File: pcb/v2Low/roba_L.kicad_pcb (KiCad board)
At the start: 2 copper layers, 10.7 x 12.1 mm, 49 parts, among them SW1 SW_PUSH, SW10 SW_PUSH, SW11 SW_PUSH, SW12 SW_PUSH, SW13 SW_PUSH, SW14 SW_PUSH, SW15 SW_PUSH, SW16 SW_PUSH, SW17 SW_PUSH, SW18 SW_PUSH, SW19 SW_PUSH, SW2 SW_PUSH, SW20 SW_PUSH, SW21 SW_PUSH, SW22 SW_PUSH, SW23 SW_PUSH, SW24 SW_SPDT, SW3 SW_PUSH, SW4 SW_PUSH, SW5 SW_PUSH, SW6 SW_PUSH, SW7 SW_PUSH, SW8 SW_PUSH, SW9 SW_PUSH

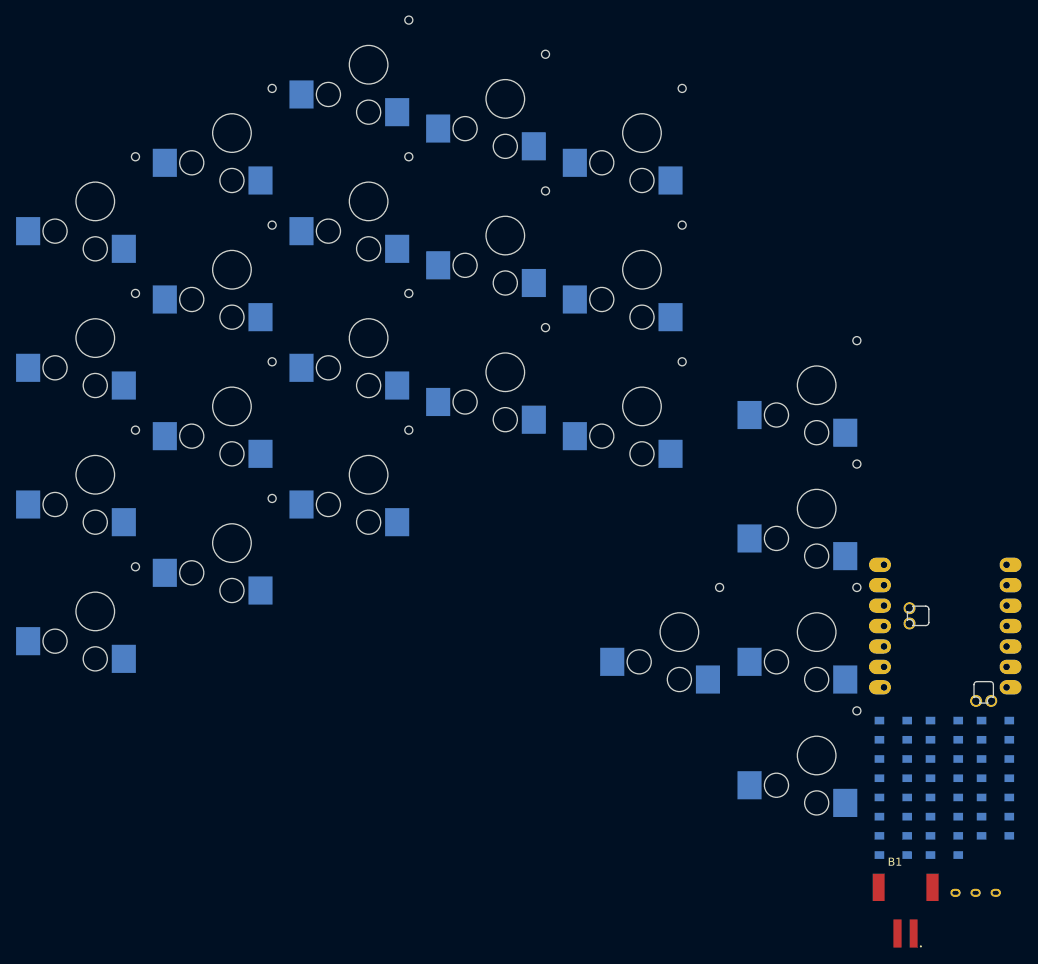
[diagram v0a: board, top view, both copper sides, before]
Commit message: save
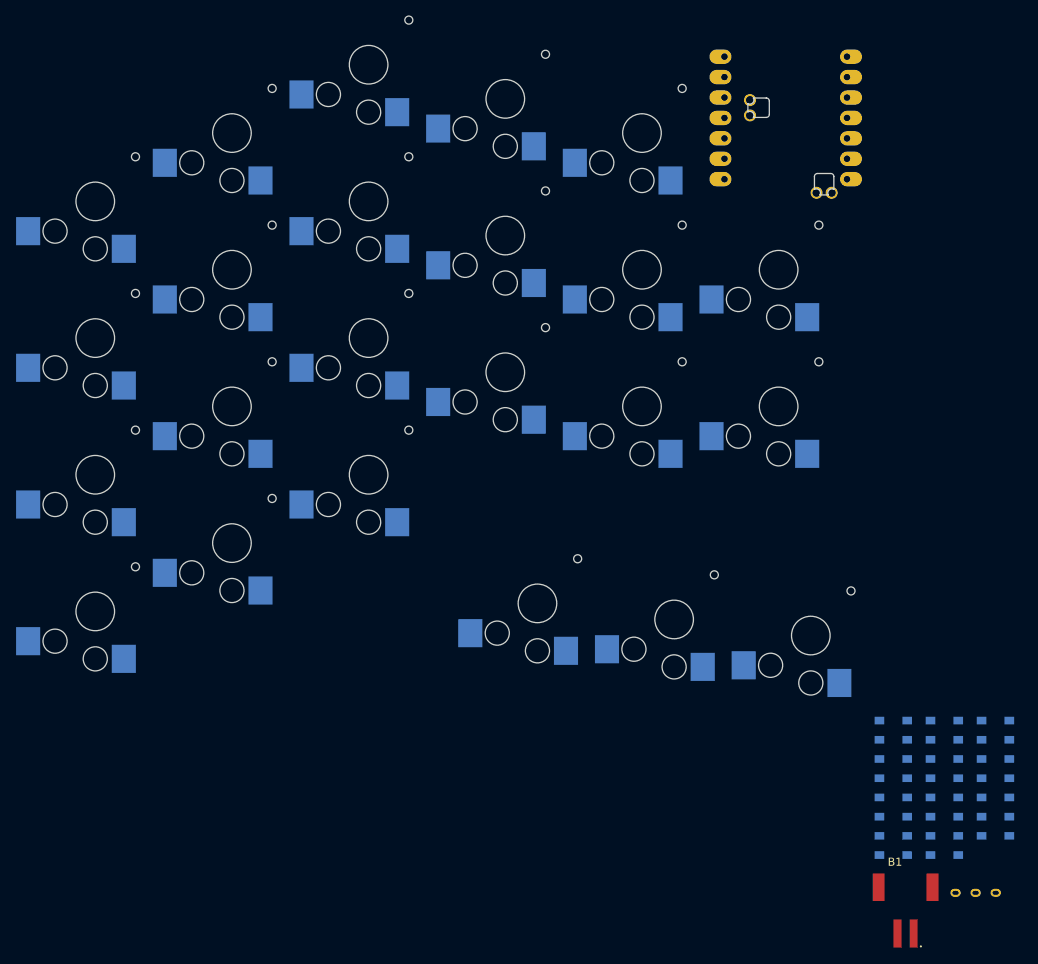
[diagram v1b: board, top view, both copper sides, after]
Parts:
- moved U1 66.2 mm to (135.9, 29.1)
- moved SW20 34.1 mm to (122.0, 102.0)
- moved SW21 30.1 mm to (135.0, 58.5)
- moved SW22 28.5 mm to (135.0, 75.5)
- moved SW16 18.0 mm to (105.0, 100.0)
- moved SW23 14.9 mm to (139.0, 104.0)
